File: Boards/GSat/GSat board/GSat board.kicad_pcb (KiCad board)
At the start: 2 copper layers, 110 x 70 mm, 25 parts, among them IC1 NEO-M8Q-0, J2 PCB.RPSMAFRA.HT, U1 TMC2209_SILENTSTEPSTICK, U12 MMBT3906-7-F, U2 TMC2209_SILENTSTEPSTICK, U3 E28-2G4M27SX, U4 E28-2G4M27SX

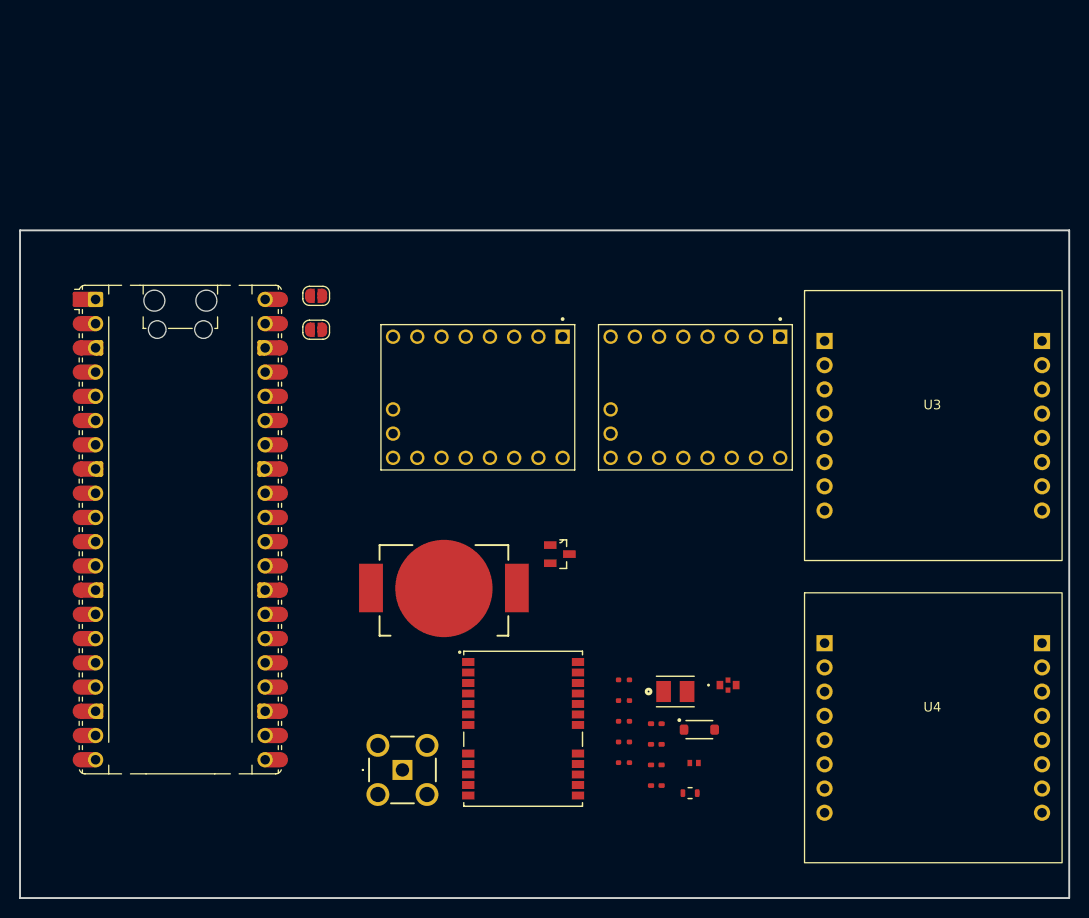
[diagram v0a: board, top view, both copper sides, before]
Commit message: GSAT (Squematic update)
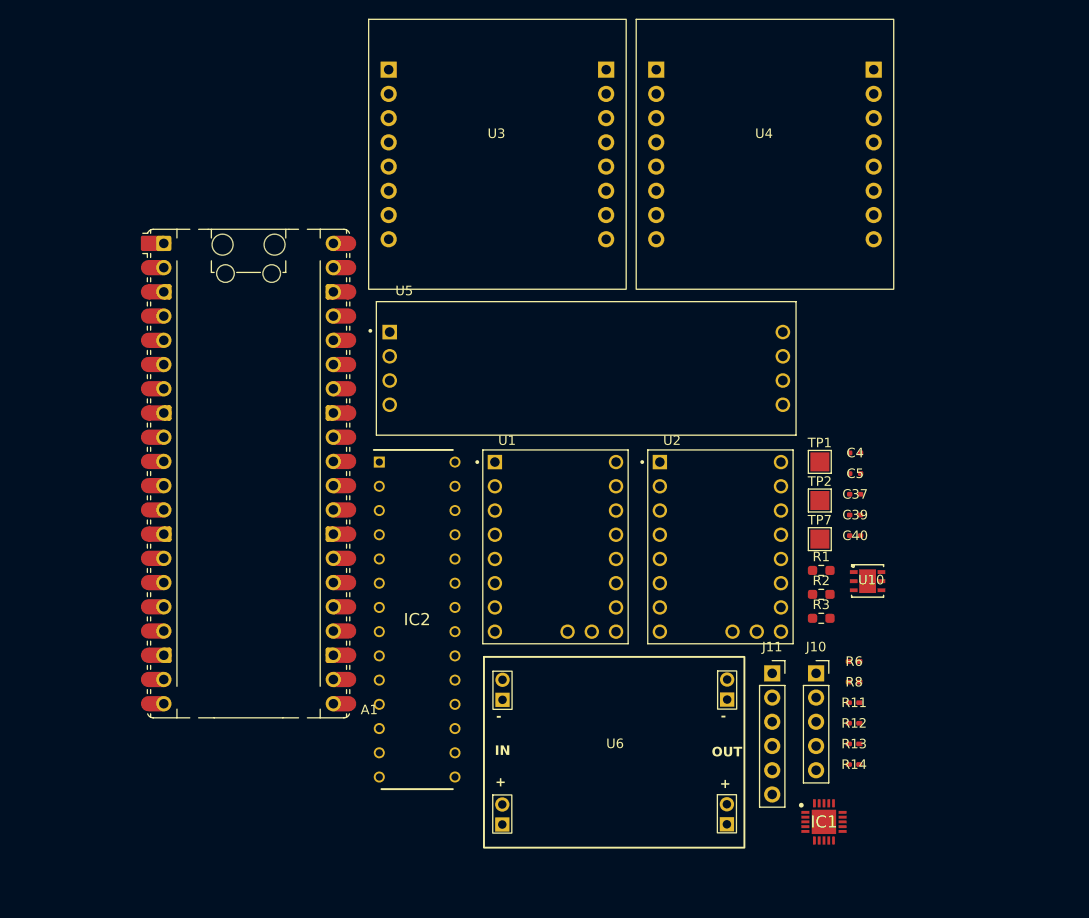
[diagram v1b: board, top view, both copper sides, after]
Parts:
- removed BT1: BAT-HLD-012-SMT-TR, BAT_HLD_012:BAT_BAT-HLD-012-SMT-TR
- removed C1: 4.7u, Capacitor-0402:Capacitor_0402
- removed C2, C3: 100n, Capacitor-0402:Capacitor_0402
- removed CR3: VLMC3100-GS08, LED-Green_VLMC3100-GS08:LED_PLCC_VSMB
- removed D2: PMEG2010ER, Diode-Schottky_PMEG2010ER:SODFL3517X110N
- removed FL1: FTCap0603, FTCap_0603:FTCap_0603
- removed J2: PCB.RPSMAFRA.HT, PCB.RPSMAFRA.HT:PCBRPSMAFRAHT
- removed JP1, JP2: Jumper_2_Open, Jumper:SolderJumper-2_P1.3mm_Open_RoundedPad1.0x1.5mm
- removed L1: 27n, Inductor-0402:Inductor_0402
- removed R10: 10k, Resistor-0402:RES_0402
- removed R5: 10, Resistor-0402:RES_0402
- removed R7: 150, Resistor-0603:RES_0603
- removed U12: MMBT3906-7-F, MMBT3906-7-F:SOT103P240X110-3N
- added C37: 4.7uF, Capacitor-0402:Capacitor_0402, F.Cu at (116.1, 84.2)
- added C39: 4.7uF, Capacitor-0402:Capacitor_0402, F.Cu at (116.1, 86.3)
- added C40: 1uF, Capacitor-0402:Capacitor_0402, F.Cu at (116.1, 88.5)
- added IC2: MCP23017-E_SP, MCP23017:DIP794W56P254L3486H508Q28N, F.Cu at (70.1, 97.3)
- added J10: Conn_01x05_Pin, Connector_PinSocket_2.54mm:PinSocket_1x05_P2.54mm_Vertical, F.Cu at (112.0, 102.9)
- added J11: Conn_01x06_Pin, Connector_PinSocket_2.54mm:PinSocket_1x06_P2.54mm_Vertical, F.Cu at (107.4, 102.9)
- added R1: 1K, Resistor_SMD:R_0603_1608Metric_Pad0.98x0.95mm_HandSolder, F.Cu at (112.5, 92.2)
- added R11: 10k, Resistor-0402:RES_0402, F.Cu at (115.9, 106.0)
- added R12: 10k, Resistor-0402:RES_0402, F.Cu at (115.9, 108.2)
- added R13: 10k, Resistor-0402:RES_0402, F.Cu at (115.9, 110.3)
- added R14: 10k, Resistor-0402:RES_0402, F.Cu at (115.9, 112.5)
- added R2: 10K, Resistor_SMD:R_0603_1608Metric_Pad0.98x0.95mm_HandSolder, F.Cu at (112.5, 94.7)
- added R3: 10K, Resistor_SMD:R_0603_1608Metric_Pad0.98x0.95mm_HandSolder, F.Cu at (112.5, 97.2)
- added TP1: TestPoint, TestPoint:TestPoint_Pad_2.0x2.0mm, F.Cu at (112.4, 80.8)
- added TP2: TestPoint, TestPoint:TestPoint_Pad_2.0x2.0mm, F.Cu at (112.4, 84.8)
- added TP7: TestPoint, TestPoint:TestPoint_Pad_2.0x2.0mm, F.Cu at (112.4, 88.9)
- added U10: ST1L05APU33R, LDO ST1L05A:DFN_5APU33R_STM, F.Cu at (117.4, 93.3)
- added U5: MAX485_MODULE_5V_LOGIC_TLL_TO_RS-485_CONVERTER, MAX485Module:MODULE_MAX485_MODULE_5V_LOGIC_TLL_TO_RS-485_CONVERTER, F.Cu at (87.9, 71.0)
- added U6: ~, DCDCModule:DCDC_Module, F.Cu at (90.9, 110.8)
- IC1: value NEO-M8Q-0 -> LTC4418IUF#PBF; footprint NEO-M8Q-0:NEO-M8_UBL -> LTC4418:QFN50P400X400X80-21N-D
- moved U4 62.7 mm to (106.6, 48.4)
- moved U3 53.8 mm to (78.6, 48.4)
- moved C4 38.8 mm to (116.1, 79.8)
- moved C5 38.8 mm to (116.1, 82.0)
- moved IC1 33.0 mm to (112.8, 118.5)
- moved U2 29.9 mm to (101.9, 89.7), turned to 0 degrees
- moved R6 22.5 mm to (115.9, 101.7)
- moved R8 22.5 mm to (115.9, 103.9)
- moved U1 21.5 mm to (84.6, 89.7), turned to 0 degrees
- moved A1 9.25 mm to (52.5, 82.0)
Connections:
- A1 pad 1: unconnected-(A1-GPIO0-Pad1) -> /GPS RX UART
- A1 pad 10: unconnected-(A1-GPIO7-Pad10) -> /I2C#2 SCL
- A1 pad 11: /LimitSwitch1 -> /RS_TX
- A1 pad 12: /LimitSwitch2 -> /RS_RX
- A1 pad 14: /LimitSwitch3 -> /UNI_BUSY
- A1 pad 15: unconnected-(A1-GPIO11-Pad15) -> /UNI_DIO1
- A1 pad 16: unconnected-(A1-GPIO12-Pad16) -> /MSD MISO
- A1 pad 17: unconnected-(A1-GPIO13-Pad17) -> /CS_MSD
- A1 pad 19: unconnected-(A1-GPIO14-Pad19) -> /MSD CLK
- A1 pad 2: unconnected-(A1-GPIO1-Pad2) -> /GPS TX UART
- A1 pad 20: unconnected-(A1-GPIO15-Pad20) -> /MSD MOSI
- A1 pad 21: unconnected-(A1-GPIO16-Pad21) -> /RADIO MISO
- A1 pad 22: /Driver1 Dir -> /CS_OMNI
- A1 pad 24: /Driver1 Step -> /RADIO CLK
- A1 pad 25: /Driver2 Dir -> /RADIO MOSI
- A1 pad 26: /Driver2 Step -> /CS_UNI
- A1 pad 27: unconnected-(A1-GPIO21-Pad27) -> /OMNI_BUSY
- A1 pad 29: unconnected-(A1-GPIO22-Pad29) -> /OMNI_DIO1
- A1 pad 34: unconnected-(A1-GPIO28_ADC2-Pad34) -> /GPS PPS
- A1 pad 35: unconnected-(A1-ADC_VREF-Pad35) -> GND
- A1 pad 4: unconnected-(A1-GPIO2-Pad4) -> /Driver1 Step
- A1 pad 5: unconnected-(A1-GPIO3-Pad5) -> /Driver2 Step
- A1 pad 6: /GPS TX UART -> /I2C#1 SDA
- A1 pad 7: /GPS RX UART -> /I2C#1 SCL
- A1 pad 9: /GPS ~{BOOT} -> /I2C#2 SDA
- IC1 pad 10: GND -> unconnected-(IC1-INTVCC-Pad10)
- IC1 pad 11: /RF -> unconnected-(IC1-G2-Pad11)
- IC1 pad 12: GND -> unconnected-(IC1-VS2-Pad12)
- IC1 pad 13: GND -> unconnected-(IC1-G1-Pad13)
- IC1 pad 20: /GPS TX UART -> unconnected-(IC1-HYS-Pad20)
- IC1 pad 21: /GPS RX UART -> unconnected-(IC1-GND_2-Pad21)
- IC1 pad 3: Net-(IC1-TIMEPULSE) -> unconnected-(IC1-OV1-Pad3)
- IC1 pad 4: /INT GPS -> unconnected-(IC1-UV2-Pad4)
- IC1 pad 7: GND -> unconnected-(IC1-~{VALID2}-Pad7)
- IC1 pad 8: /GPS ~{BOOT} -> unconnected-(IC1-GND_1-Pad8)
- IC1 pad 9: Net-(IC1-VCC_RF) -> unconnected-(IC1-CAS-Pad9)
- U1 pad 14: +3.3V -> /Driver1 MS2
- U1 pad 15: +3.3V -> /Driver1 MS1
- U2 pad 14: +3.3V -> /Driver2 MS2
- U2 pad 15: +3.3V -> /Driver2 MS1
- U3 pad 10: unconnected-(U3-GND-Pad10) -> GND
- U3 pad 11: unconnected-(U3-NRESET-Pad11) -> /UNI_NRESET
- U3 pad 12: unconnected-(U3-BUSY-Pad12) -> /UNI_BUSY
- U3 pad 13: unconnected-(U3-DIO1-Pad13) -> /UNI_DIO1
- U3 pad 16: unconnected-(U3-GND-Pad16) -> GND
- U3 pad 3: /MISO -> /RADIO MISO
- U3 pad 4: /MOSI -> /RADIO MOSI
- U3 pad 5: /CLK -> /RADIO CLK
- U3 pad 6: /CS -> /CS_UNI
- U3 pad 8: /ANT_RX_EN -> /UNI_RX_EN
- U3 pad 9: unconnected-(U3-TX_EN-Pad9) -> /UNI_TX_EN
- U4 pad 10: unconnected-(U4-GND-Pad10) -> GND
- U4 pad 11: unconnected-(U4-NRESET-Pad11) -> /OMNI_NRESET
- U4 pad 12: unconnected-(U4-BUSY-Pad12) -> /OMNI_BUSY
- U4 pad 13: unconnected-(U4-DIO1-Pad13) -> /OMNI_DIO1
- U4 pad 16: unconnected-(U4-GND-Pad16) -> GND
- U4 pad 3: /MISO -> /RADIO MISO
- U4 pad 4: /MOSI -> /RADIO MOSI
- U4 pad 5: /CLK -> /RADIO CLK
- U4 pad 6: /CS -> /CS_OMNI
- U4 pad 8: /ANT_RX_EN -> /OMNI_RX_EN
- U4 pad 9: unconnected-(U4-TX_EN-Pad9) -> /OMNI_TX_EN
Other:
- board outline removed
